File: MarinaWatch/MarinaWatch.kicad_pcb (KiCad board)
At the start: 2 copper layers, 54 x 32 mm, 8 parts, among them J1 USB_C_Receptacle_USB2.0_16P, U1 ESP32-S3-WROOM-1

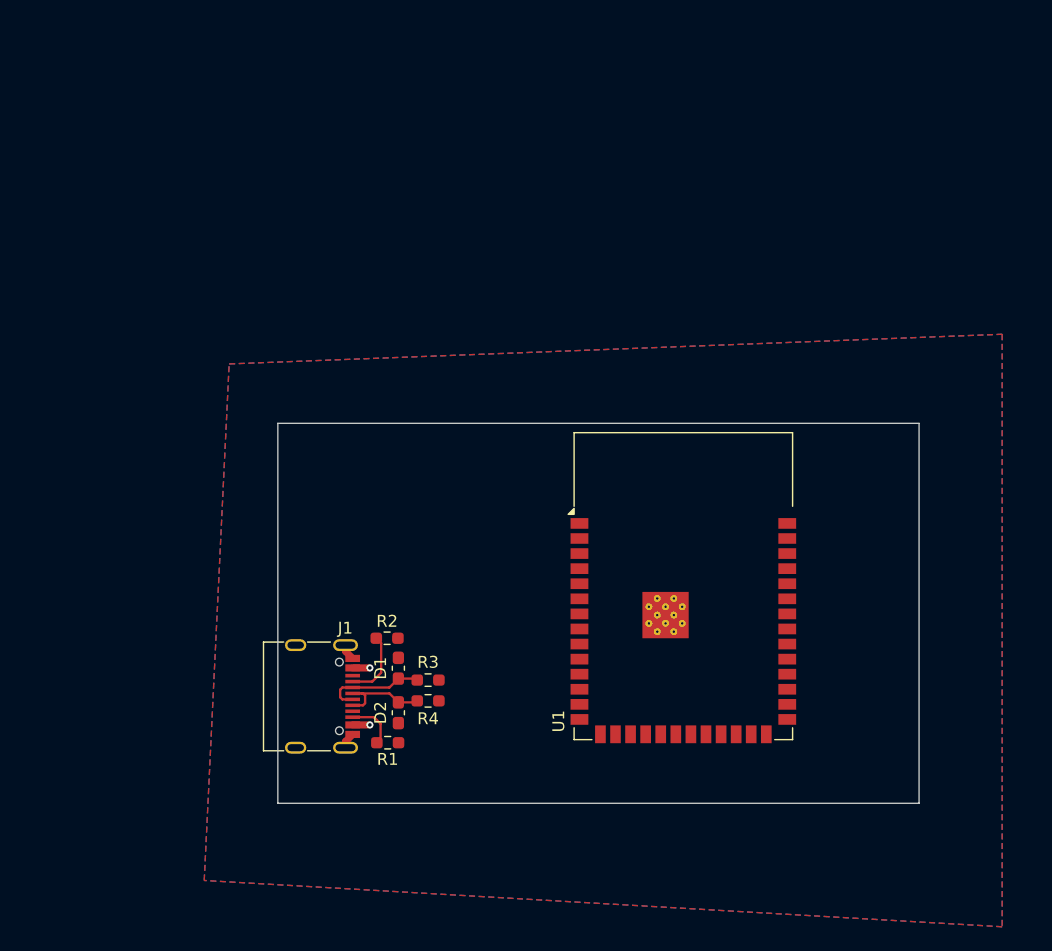
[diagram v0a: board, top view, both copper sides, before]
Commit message: Structure power supply chain
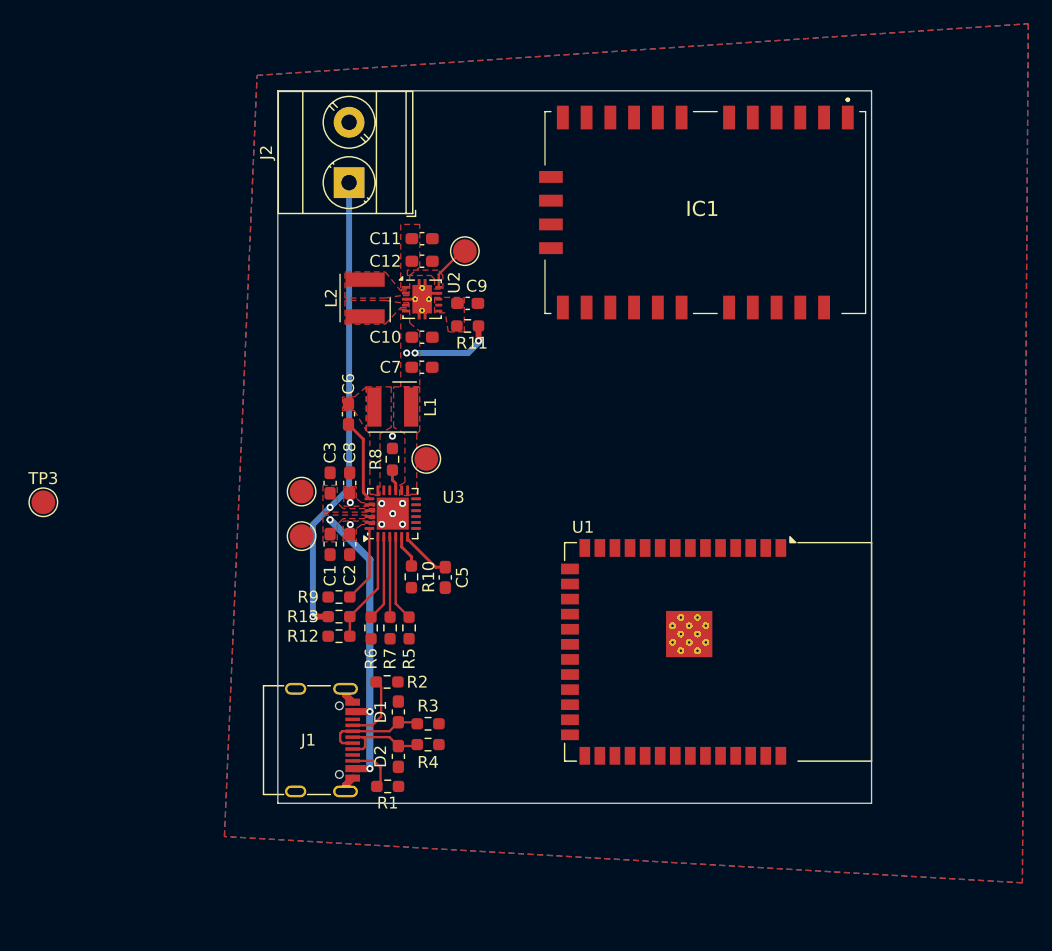
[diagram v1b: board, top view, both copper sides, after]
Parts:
- added C1: 1u, Capacitor_SMD:C_0603_1608Metric_Pad1.08x0.95mm_HandSolder, F.Cu at (104.4, 78.2)
- added C10: 10u, Capacitor_SMD:C_0603_1608Metric_Pad1.08x0.95mm_HandSolder, F.Cu at (112.2, 60.8)
- added C11: 10u, Capacitor_SMD:C_0603_1608Metric_Pad1.08x0.95mm_HandSolder, F.Cu at (112.2, 52.5)
- added C12: 10u, Capacitor_SMD:C_0603_1608Metric_Pad1.08x0.95mm_HandSolder, F.Cu at (112.2, 54.4)
- added C2: 1u, Capacitor_SMD:C_0603_1608Metric_Pad1.08x0.95mm_HandSolder, F.Cu at (106.0, 78.2)
- added C3: 1u, Capacitor_SMD:C_0603_1608Metric_Pad1.08x0.95mm_HandSolder, F.Cu at (104.4, 73.0)
- added C5: 1u, Capacitor_SMD:C_0603_1608Metric_Pad1.08x0.95mm_HandSolder, F.Cu at (114.1, 81.0)
- added C6: 1u, Capacitor_SMD:C_0603_1608Metric_Pad1.08x0.95mm_HandSolder, F.Cu at (106.0, 67.2)
- added C7: 1u, Capacitor_SMD:C_0603_1608Metric_Pad1.08x0.95mm_HandSolder, F.Cu at (112.1, 63.3)
- added C8: 4u7, Capacitor_SMD:C_0603_1608Metric_Pad1.08x0.95mm_HandSolder, F.Cu at (106.0, 73.0)
- added C9: 100n, Capacitor_SMD:C_0603_1608Metric_Pad1.08x0.95mm_HandSolder, F.Cu at (116.0, 57.9)
- added IC1: 2609011181000, Lund Formula Student:2609011181000, F.Cu at (136.0, 50.2)
- added J2: Screw_Terminal_01x02, TerminalBlock_Phoenix:TerminalBlock_Phoenix_MKDS-3-2-5.08_1x02_P5.08mm_Horizontal, F.Cu at (106.0, 47.7)
- added L1: 2u2, Inductor_SMD_Wurth:L_Wurth_WE-LQSH-4020, F.Cu at (109.7, 66.6)
- added L2: 2u2, Inductor_SMD_Wurth:L_Wurth_WE-LQSH-4020, F.Cu at (107.3, 57.5)
- added R10: 1k, Resistor_SMD:R_0603_1608Metric_Pad0.98x0.95mm_HandSolder, F.Cu at (111.2, 80.9)
- added R11: 100R, Resistor_SMD:R_0603_1608Metric_Pad0.98x0.95mm_HandSolder, F.Cu at (116.0, 59.8)
- added R12: 10k, Resistor_SMD:R_0603_1608Metric_Pad0.98x0.95mm_HandSolder, F.Cu at (105.2, 85.9)
- added R13: 27k, Resistor_SMD:R_0603_1608Metric_Pad0.98x0.95mm_HandSolder, F.Cu at (105.2, 84.3)
- added R5: 10k, Resistor_SMD:R_0603_1608Metric_Pad0.98x0.95mm_HandSolder, F.Cu at (111.0, 85.2)
- added R6: 10k, Resistor_SMD:R_0603_1608Metric_Pad0.98x0.95mm_HandSolder, F.Cu at (107.8, 85.2)
- added R7: 10k, Resistor_SMD:R_0603_1608Metric_Pad0.98x0.95mm_HandSolder, F.Cu at (109.5, 85.2)
- added R8: 10k, Resistor_SMD:R_0603_1608Metric_Pad0.98x0.95mm_HandSolder, F.Cu at (109.7, 71.0)
- added R9: 10k, Resistor_SMD:R_0603_1608Metric_Pad0.98x0.95mm_HandSolder, F.Cu at (105.2, 82.6)
- added TP1: TestPoint, TestPoint:TestPoint_Pad_D2.0mm, F.Cu at (102.0, 77.5)
- added TP2: TestPoint, TestPoint:TestPoint_Pad_D2.0mm, F.Cu at (102.0, 73.8)
- added TP3: TestPoint, TestPoint:TestPoint_Pad_D2.0mm, F.Cu at (80.2, 74.7)
- added TP4: TestPoint, TestPoint:TestPoint_Pad_D2.0mm, F.Cu at (112.5, 71.0)
- added TP5: TestPoint, TestPoint:TestPoint_Pad_D2.0mm, F.Cu at (115.8, 53.5)
- added U2: TPS63001, Package_SON:Texas_DRC0010J_ThermalVias, F.Cu at (112.2, 57.5)
- added U3: BQ24166RGE, Package_DFN_QFN:Texas_RGE0024H_VQFN-24-1EP_4x4mm_P0.5mm_EP2.7x2.7mm, F.Cu at (109.7, 75.6)
- moved U1 6.29 mm to (137.1, 87.2), turned to -90 degrees
- moved D1 3.68 mm to (110.2, 92.3)
- moved D2 3.68 mm to (110.2, 96.1)
- moved J1 3.68 mm to (102.6, 94.7)
- moved R2 3.68 mm to (109.2, 89.8)
- moved R3 3.68 mm to (112.7, 93.3)
- moved R4 3.68 mm to (112.7, 95.1)
- moved R1 3.68 mm to (109.2, 98.6)
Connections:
- U1 pad 2: unconnected-(U1-3V3-Pad2) -> +3.3V
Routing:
- net VDD: track 0.00 -> 39.1 mm, vias 0 -> 2
- net VBUS: track 2.90 -> 25.2 mm, vias 2 -> 3
- net /VDPM: track 0.00 -> 9.34 mm
- net /IUSB1: track 0.00 -> 7.22 mm
- net /IUSB3: track 0.00 -> 7.20 mm
- net VCC: track 0.00 -> 7.11 mm, vias 0 -> 3
- net /BOOT: track 0.00 -> 6.99 mm
- net /IUSB2: track 0.00 -> 6.76 mm
- net /CE: track 0.00 -> 6.46 mm
- net /DRV: track 0.00 -> 4.34 mm
- net +3.3V: track 0.00 -> 4.11 mm
- net /ISET: track 0.00 -> 2.79 mm
- net GND: track 2.74 -> 5.17 mm, vias 0 -> 6
- net /ILIM: track 0.00 -> 1.81 mm
- net /PMIDU: vias 0 -> 1
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- added copper zone on F.Cu, net +3.3V
- added copper zone on F.Cu, net /L1
- added copper zone on F.Cu, net /L2
- added copper zone on F.Cu, net /PMIDI
- added copper zone on F.Cu, net /PMIDU
- added copper zone on F.Cu, net /SW
- added copper zone on F.Cu, net /VINA
- added copper zone on F.Cu, net VBUS
- added copper zone on F.Cu, net VCC
- added copper zone on F.Cu, net VDD
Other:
- board size 54 x 32 mm -> 50 x 60 mm
